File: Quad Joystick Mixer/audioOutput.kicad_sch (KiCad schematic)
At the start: 30 parts, among them J2 NMJ6HCD, U4 OPA1692xD

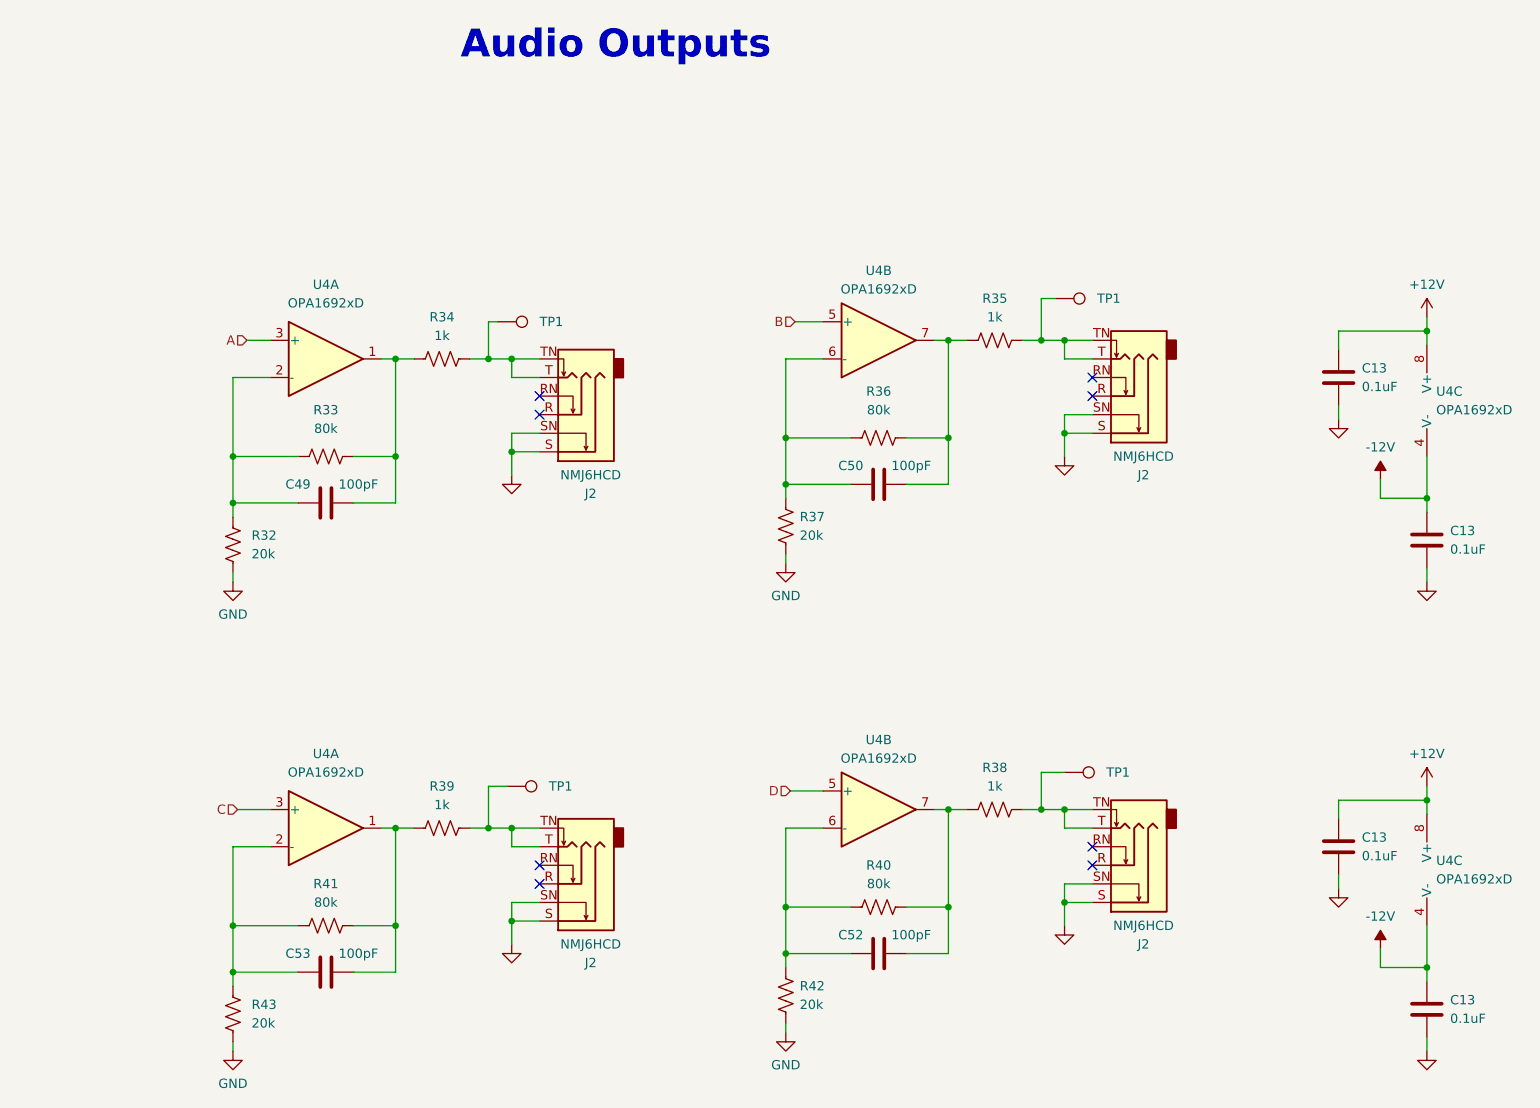
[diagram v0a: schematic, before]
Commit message: clean up after review, working through BOM
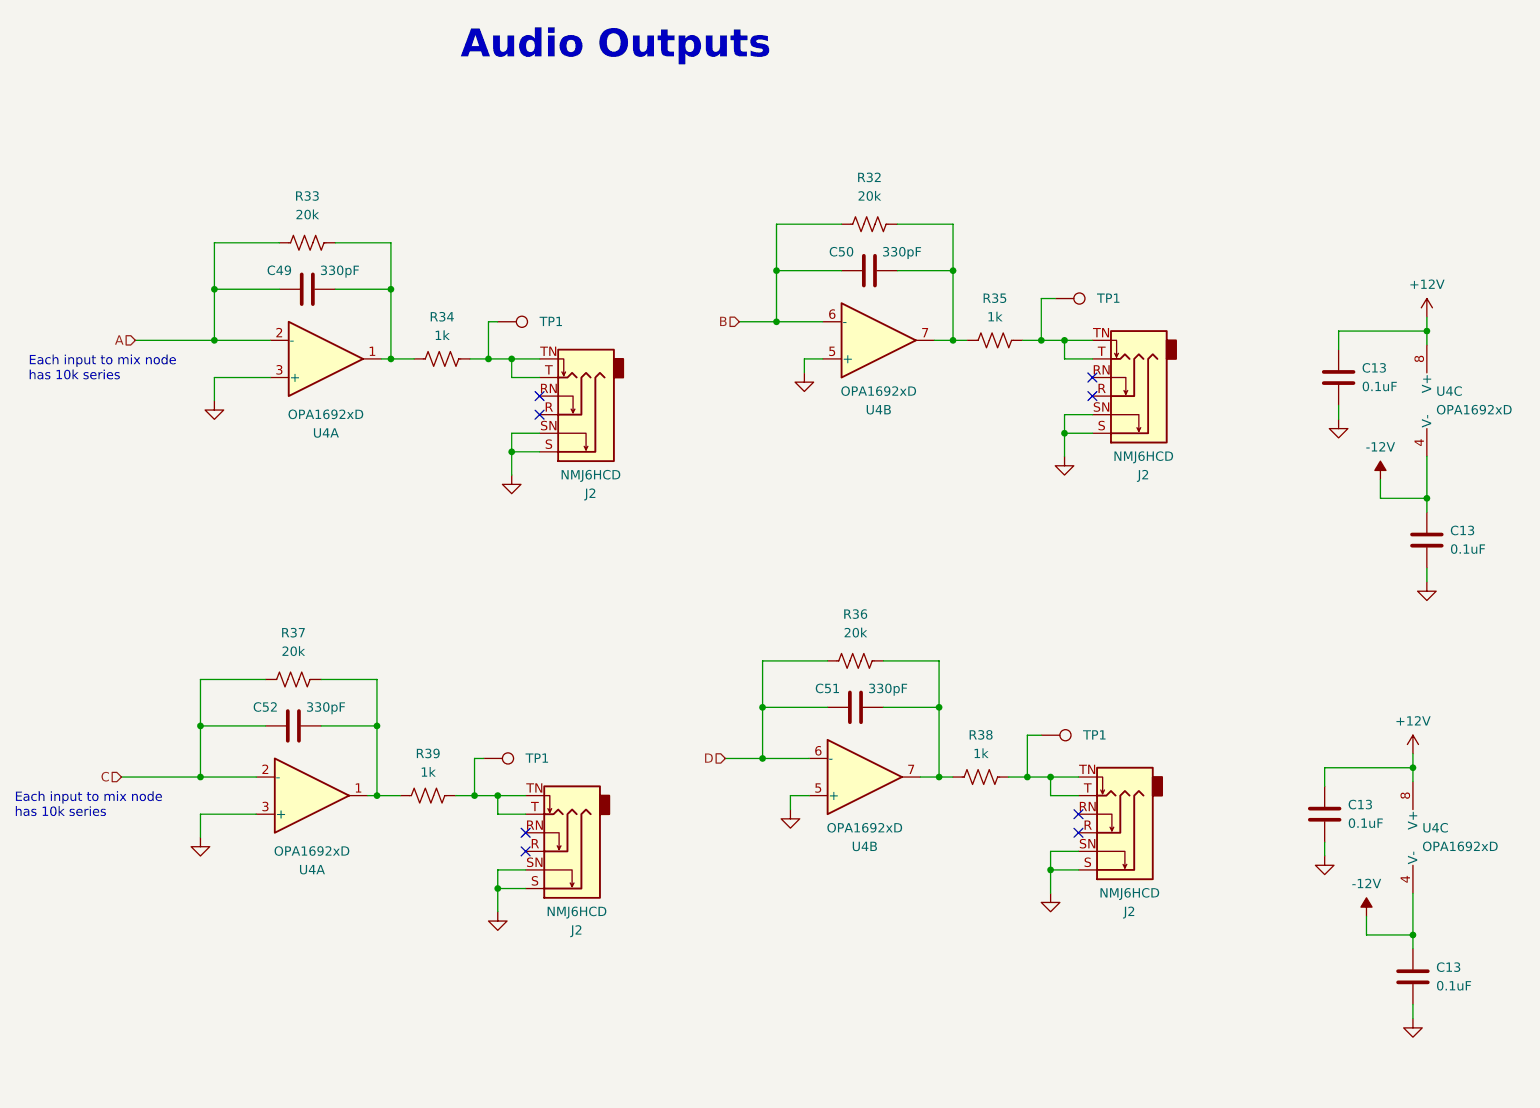
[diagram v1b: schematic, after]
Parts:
- removed C13 (x2): 0.1uF, Capacitor_SMD:C_0805_2012Metric_Pad1.18x1.45mm_HandSolder, symbol Device:C
- removed C53: 100pF, symbol Device:C
- removed J2 (x2): NMJ6HCD, Eyewool Connectors:NMJ6HCD, symbol Connector_Audio:AudioJack3_Switch
- removed R40, R41: 80k, symbol Device:R_US
- removed R42, R43: 20k, symbol Device:R_US
- removed TP1 (x2): TestPoint, TestPoint:TestPoint_THTPad_D1.5mm_Drill0.7mm, symbol Connector:TestPoint
- added C13 (x2): 0.1uF, Capacitor_SMD:C_0805_2012Metric_Pad1.18x1.45mm_HandSolder, symbol Device:C
- added C51: 330pF, Capacitor_SMD:C_0805_2012Metric_Pad1.18x1.45mm_HandSolder, symbol Device:C
- added J2 (x2): NMJ6HCD, Eyewool Connectors:NMJ6HCD, symbol Connector_Audio:AudioJack3_Switch
- added TP1 (x2): TestPoint, TestPoint:TestPoint_THTPad_D1.5mm_Drill0.7mm, symbol Connector:TestPoint
- C49, C50, C52: value 100pF -> 330pF; footprint (none) -> Capacitor_SMD:C_0805_2012Metric_Pad1.18x1.45mm_HandSolder; DK PN (none) -> 399-C0805C331J5GAC7800CT-ND; MPN (none) -> C0805C331J5GAC7800
- R33, R36: value 80k -> 20k
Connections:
- net +12V: now also C13.1
- net -12V: now also C13.1
- net A: now also C49.1, R33.2, U4.2 (-); no longer U4.3 (+)
- net B: now also C50.1, R32.2, U4.6 (-); no longer U4.5 (+)
- net C: now also C52.1, R37.2, U4.2 (-); no longer U4.3 (+)
- net D: now also R36.2, U4.6 (-), C51.1; no longer U4.5 (+)
- net GND: now also U4.3 (+), U4.3 (+), U4.5 (+), U4.5 (+), C13.2, C13.2, J2.S, J2.S, J2.SN, J2.SN; no longer R32.2, R37.2
- net at R38.1: now also J2.T, J2.TN, TP1.1
- net at R39.1: now also J2.T, J2.TN, TP1.1
- net at R39.2, U4.1: now also C52.2, R37.1
- net at R38.2, U4.7: now also R36.1, C51.2; no longer C52.2
- net at C50.2, R35.2, U4.7: now also R32.1; no longer R36.1
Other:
- note added: "Each input to mix node has 10k series"
- moved on the sheet: C49, R33
